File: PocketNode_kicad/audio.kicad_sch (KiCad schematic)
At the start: 16 parts, among them J3 AudioPlug3, U4 PCM5102APWR, U5 NJM2073M-ND

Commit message: update
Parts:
- C10, C11, C12, C13, C14, C15, C16, C17, C20, C21, C22: footprint (none) -> Capacitor_SMD:C_0603_1608Metric_Pad1.08x0.95mm_HandSolder
- C18, C19: footprint (none) -> Capacitor_SMD:C_0805_2012Metric_Pad1.18x1.45mm_HandSolder
- U4: footprint PCM5102APWR -> Library:SOP65P640X120-20N
- U5: footprint NJR-DMP8_NJR -> Library:NJR-DMP8_NJR
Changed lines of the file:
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@@
 			)
 		)
-		(property "Footprint" ""
+		(property "Footprint" "Capacitor_SMD:C_0603_1608Metric_Pad1.08x0.95mm_HandSolder"
 			(at 67.31 41.91 0)
 			(effects
@@
 			)
 		)
-		(property "Footprint" ""
+		(property "Footprint" "Capacitor_SMD:C_0805_2012Metric_Pad1.18x1.45mm_HandSolder"
 			(at 170.18 30.48 0)
 			(effects
@@
 			)
 		)
-		(property "Footprint" ""
+		(property "Footprint" "Capacitor_SMD:C_0603_1608Metric_Pad1.08x0.95mm_HandSolder"
 			(at 55.88 31.75 0)
 			(effects
@@
 			)
 		)
-		(property "Footprint" "NJR-DMP8_NJR"
+		(property "Footprint" "Library:NJR-DMP8_NJR"
 			(at 179.07 33.02 0)
 			(effects
@@
 			)
 		)
-		(property "Footprint" ""
+		(property "Footprint" "Capacitor_SMD:C_0603_1608Metric_Pad1.08x0.95mm_HandSolder"
 			(at 67.31 31.75 0)
 			(effects
@@
 			)
 		)
-		(property "Footprint" ""
+		(property "Footprint" "Capacitor_SMD:C_0603_1608Metric_Pad1.08x0.95mm_HandSolder"
 			(at 128.27 54.61 0)
 			(effects
@@
 			)
 		)
-		(property "Footprint" ""
+		(property "Footprint" "Capacitor_SMD:C_0603_1608Metric_Pad1.08x0.95mm_HandSolder"
 			(at 55.88 41.91 0)
 			(effects
@@
 			)
 		)
-		(property "Footprint" "PCM5102APWR"
+		(property "Footprint" "Library:SOP65P640X120-20N"
 			(at 105.41 59.69 0)
 			(effects
@@
 			)
 		)
-		(property "Footprint" ""
+		(property "Footprint" "Capacitor_SMD:C_0603_1608Metric_Pad1.08x0.95mm_HandSolder"
 			(at 128.27 62.23 0)
 			(effects
@@
 			)
 		)
-		(property "Footprint" ""
+		(property "Footprint" "Capacitor_SMD:C_0603_1608Metric_Pad1.08x0.95mm_HandSolder"
 			(at 78.74 34.29 0)
 			(effects
@@
 			)
 		)
-		(property "Footprint" ""
+		(property "Footprint" "Capacitor_SMD:C_0603_1608Metric_Pad1.08x0.95mm_HandSolder"
 			(at 152.4 38.1 0)
 			(effects
@@
 			)
 		)
-		(property "Footprint" ""
+		(property "Footprint" "Capacitor_SMD:C_0603_1608Metric_Pad1.08x0.95mm_HandSolder"
 			(at 142.24 38.1 0)
 			(effects
@@
 			)
 		)
-		(property "Footprint" ""
+		(property "Footprint" "Capacitor_SMD:C_0805_2012Metric_Pad1.18x1.45mm_HandSolder"
 			(at 170.18 45.72 0)
 			(effects
@@
 			)
 		)
-		(property "Footprint" ""
+		(property "Footprint" "Capacitor_SMD:C_0603_1608Metric_Pad1.08x0.95mm_HandSolder"
 			(at 77.47 44.45 0)
 			(effects
@@
 			)
 		)
-		(property "Footprint" ""
+		(property "Footprint" "Capacitor_SMD:C_0603_1608Metric_Pad1.08x0.95mm_HandSolder"
 			(at 132.08 69.85 0)
 			(effects

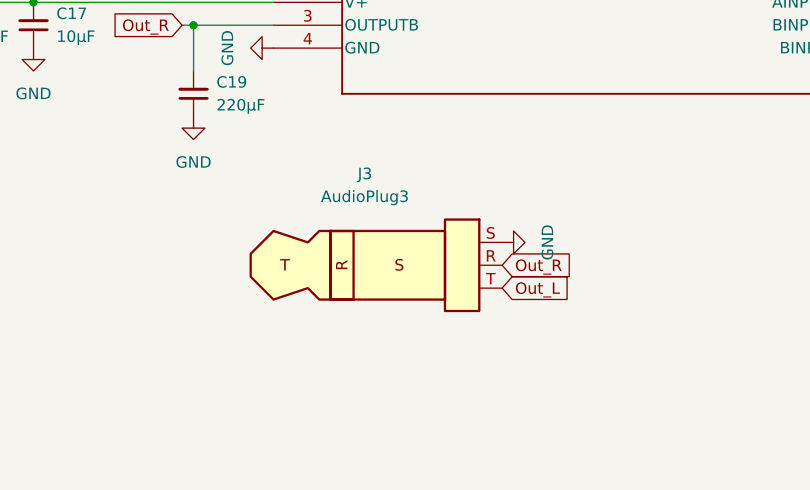
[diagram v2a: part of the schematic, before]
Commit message: update
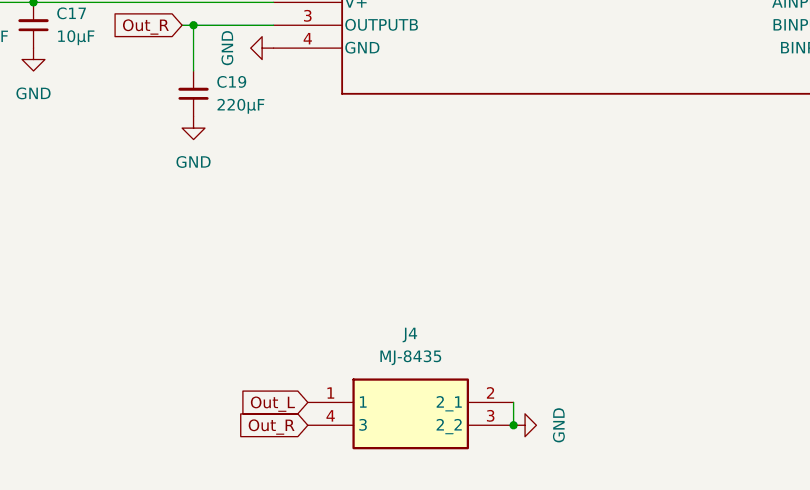
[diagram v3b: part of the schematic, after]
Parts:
- removed J3: AudioPlug3, symbol Connector_Audio:AudioPlug3
- added J4: MJ-8435, Library:MJ-8435, symbol Library:MJ-8435
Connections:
- net GND: now also J4.2 (2_1), J4.3 (2_2)
- net Out_L: now also J4.1
- net Out_R: now also J4.4 (3)
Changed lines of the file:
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@@
 	(paper "A4")
 	(junction
+		(at 205.74 82.55)
+		(diameter 0)
+		(color 0 0 0 0)
+	)
+	(junction
 		(at 128.27 57.15)
 		(diameter 0)
@@
 	(wire
 		(pts
+			(xy 205.74 80.01) (xy 205.74 82.55)
+		)
+		(stroke
+			(width 0)
+			(type default)
+		)
+	)
+	(wire
+		(pts
 			(xy 142.24 35.56) (xy 152.4 35.56)
 		)
@@
 		)
 	)
-	(global_label "Out_R"
-		(shape input)
-		(at 204.47 64.77 0)
-		(fields_autoplaced yes)
-		(effects
-			(font
-				(size 1.27 1.27)
-			)
-			(justify left)
-		)
-		(property "Intersheetrefs" "${INTERSHEET_REFS}"
-			(at 212.898 64.77 0)
-			(effects
-				(font
-					(size 1.27 1.27)
-				)
-				(justify left)
-				(hide yes)
-			)
-		)
-	)
 	(global_label "+3.3V"
 		(shape input)
@@
 		)
 	)
-	(global_label "Out_L"
+	(global_label "+3.3V"
 		(shape input)
-		(at 204.47 67.31 0)
+		(at 50.8 39.37 180)
 		(fields_autoplaced yes)
 		(effects
@@
 				(size 1.27 1.27)
 			)
-			(justify left)
+			(justify right)
 		)
 		(property "Intersheetrefs" "${INTERSHEET_REFS}"
-			(at 212.6561 67.31 0)
+			(at 42.13 39.37 0)
 			(effects
 				(font
 					(size 1.27 1.27)
 				)
-				(justify left)
+				(justify right)
 				(hide yes)
 			)
 		)
 	)
-	(global_label "+3.3V"
+	(global_label "Out_R"
 		(shape input)
-		(at 50.8 39.37 180)
+		(at 182.88 82.55 180)
 		(fields_autoplaced yes)
 		(effects
@@
 		)
 		(property "Intersheetrefs" "${INTERSHEET_REFS}"
-			(at 42.13 39.37 0)
+			(at 174.452 82.55 0)
 			(effects
 				(font
@@
 		)
 	)
+	(global_label "Out_L"
+		(shape input)
+		(at 182.88 80.01 180)
+		(fields_autoplaced yes)
+		(effects
+			(font
+				(size 1.27 1.27)
+			)
+			(justify right)
+		)
+		(property "Intersheetrefs" "${INTERSHEET_REFS}"
+			(at 174.6939 80.01 0)
+			(effects
+				(font
+					(size 1.27 1.27)
+				)
+				(justify right)
+				(hide yes)
+			)
+		)
+	)
 	(symbol
 		(lib_id "Device:C_Small")
@@
 	)
 	(symbol
-		(lib_id "Connector_Audio:AudioPlug3")
-		(at 189.23 64.77 0)
+		(lib_id "Library:MJ-8435")
+		(at 182.88 80.01 0)
 		(unit 1)
 		(exclude_from_sim no)
@@
 		(dnp no)
 		(fields_autoplaced yes)
-		(property "Reference" "J3"
-			(at 189.23 54.61 0)
+		(property "Reference" "J4"
+			(at 194.31 72.39 0)
 			(effects
 				(font
@@
 			)
 		)
-		(property "Value" "AudioPlug3"
-			(at 189.23 57.15 0)
+		(property "Value" "MJ-8435"
+			(at 194.31 74.93 0)
 			(effects
 				(font
@@
 			)
 		)
-		(property "Footprint" ""
-			(at 191.77 66.04 0)
+		(property "Footprint" "Library:MJ-8435"
+			(at 201.93 174.93 0)
 			(effects
 				(font
 					(size 1.27 1.27)
 				)
+				(justify left top)
 				(hide yes)
 			)
 		)
-		(property "Datasheet" "~"
-			(at 191.77 66.04 0)
+		(property "Datasheet" "http://akizukidenshi.com/download/ds/marushin/mj8435.pdf"
+			(at 201.93 274.93 0)
 			(effects
 				(font
 					(size 1.27 1.27)
 				)
+				(justify left top)
 				(hide yes)
 			)
 		)
-		(property "Description" "Audio Jack, 3 Poles (Stereo / TRS)"
-			(at 189.23 64.77 0)
+		(property "Description" "3.5 earphone jack"
+			(at 182.88 80.01 0)
 			(effects
 				(font
@@
 			)
 		)
-		(pin "S"
+		(property "Height" ""
+			(at 201.93 474.93 0)
+			(effects
+				(font
+					(size 1.27 1.27)
+				)
+				(justify left top)
+				(hide yes)
+			)
+		)
+		(property "Manufacturer_Name" "Marushin Electric"
+			(at 201.93 574.93 0)
+			(effects
+				(font
+					(size 1.27 1.27)
+				)
+				(justify left top)
+				(hide yes)
+			)
 		)
-		(pin "R"
+		(property "Manufacturer_Part_Number" "MJ-8435"
+			(at 201.93 674.93 0)
+			(effects
+				(font
+					(size 1.27 1.27)
+				)
+				(justify left top)
+				(hide yes)
+			)
 		)
-		(pin "T"
+		(property "Mouser Part Number" ""
+			(at 201.93 774.93 0)
+			(effects
+				(font
+					(size 1.27 1.27)
+				)
+				(justify left top)
+				(hide yes)
+			)
+		)
+		(property "Mouser Price/Stock" ""
+			(at 201.93 874.93 0)
+			(effects
+				(font
+					(size 1.27 1.27)
+				)
+				(justify left top)
+				(hide yes)
+			)
+		)
+		(property "Arrow Part Number" ""
+			(at 201.93 974.93 0)
+			(effects
+				(font
+					(size 1.27 1.27)
+				)
+				(justify left top)
+				(hide yes)
+			)
+		)
+		(property "Arrow Price/Stock" ""
+			(at 201.93 1074.93 0)
+			(effects
+				(font
+					(size 1.27 1.27)
+				)
+				(justify left top)
+				(hide yes)
+			)
+		)
+		(pin "4"
+		)
+		(pin "1"
+		)
+		(pin "2"
+		)
+		(pin "3"
 		)
 		(instances
 			(project ""
 				(path "/e2b3b76c-15d2-45d4-9847-56ef7109e38b/774ade8b-4e58-45a4-b72f-045587259432"
-					(reference "J3")
+					(reference "J4")
 					(unit 1)
 				)
@@
 	(symbol
 		(lib_id "power:GND")
-		(at 204.47 62.23 90)
+		(at 205.74 82.55 90)
 		(unit 1)
 		(exclude_from_sim no)
@@
 		(dnp no)
 		(property "Reference" "#PWR042"
-			(at 210.82 62.23 0)
+			(at 212.09 82.55 0)
 			(effects
 				(font
@@
 		)
 		(property "Value" "GND"
-			(at 209.55 62.23 0)
+			(at 210.82 82.55 0)
 			(effects
 				(font
@@
 		)
 		(property "Footprint" ""
-			(at 204.47 62.23 0)
+			(at 205.74 82.55 0)
 			(effects
 				(font
@@
 		)
 		(property "Datasheet" ""
-			(at 204.47 62.23 0)
+			(at 205.74 82.55 0)
 			(effects
 				(font
@@
 		)
 		(property "Description" "Power symbol creates a global label with name \"GND\" , ground"
-			(at 204.47 62.23 0)
+			(at 205.74 82.55 0)
 			(effects
 				(font
